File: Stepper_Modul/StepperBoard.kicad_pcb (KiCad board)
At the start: 2 copper layers, 55.1 x 100 mm, 67 parts, among them J101 Screw_Terminal_01x02, J102 Screw_Terminal_01x04, J103 Screw_Terminal_01x04, J104 Screw_Terminal_01x04, J105 Screw_Terminal_01x04, J106 Conn_02x20_Odd_Even, SW201 SW_DIP_x03, SW401 SW_DIP_x03, SW501 SW_DIP_x03, SW502 SW_DIP_x03, U201 TMC2226, U401 TMC2226, U501 TMC2226, U502 TMC2226

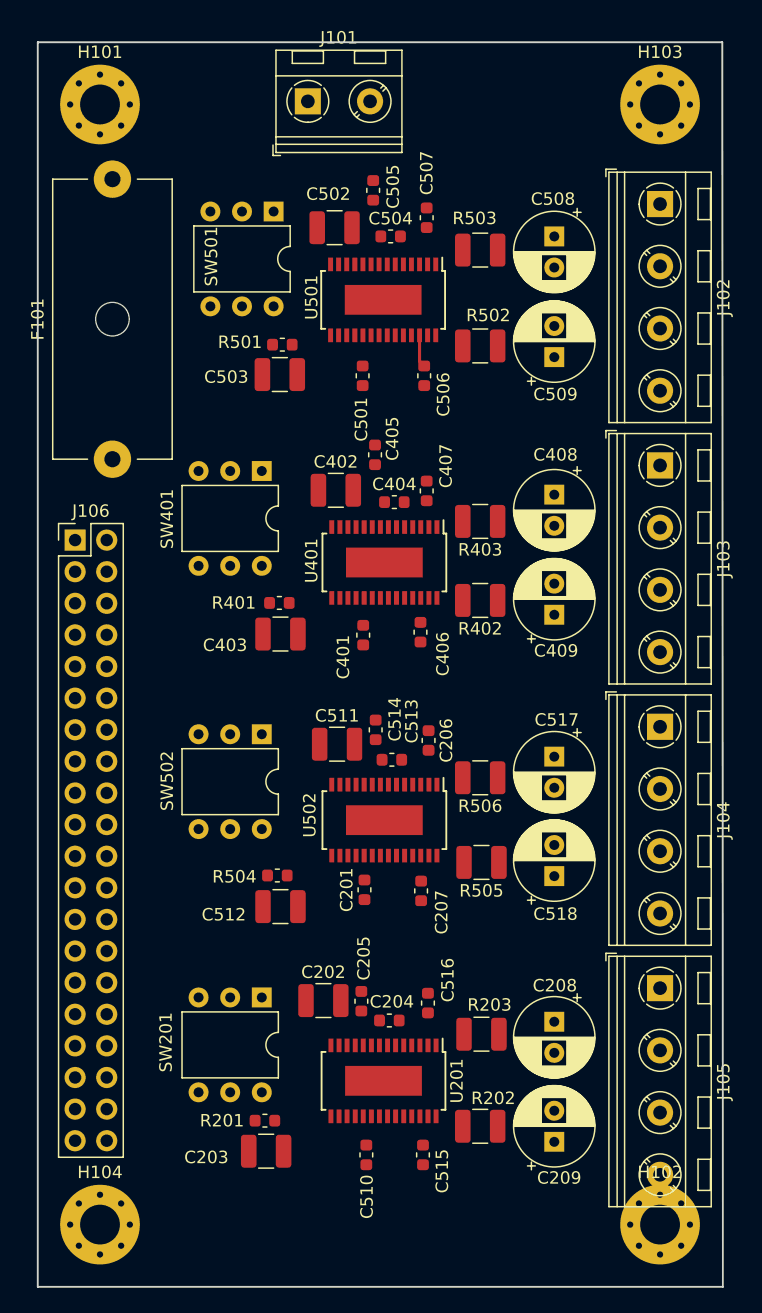
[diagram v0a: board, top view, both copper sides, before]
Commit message: stepper board fertig gestellt
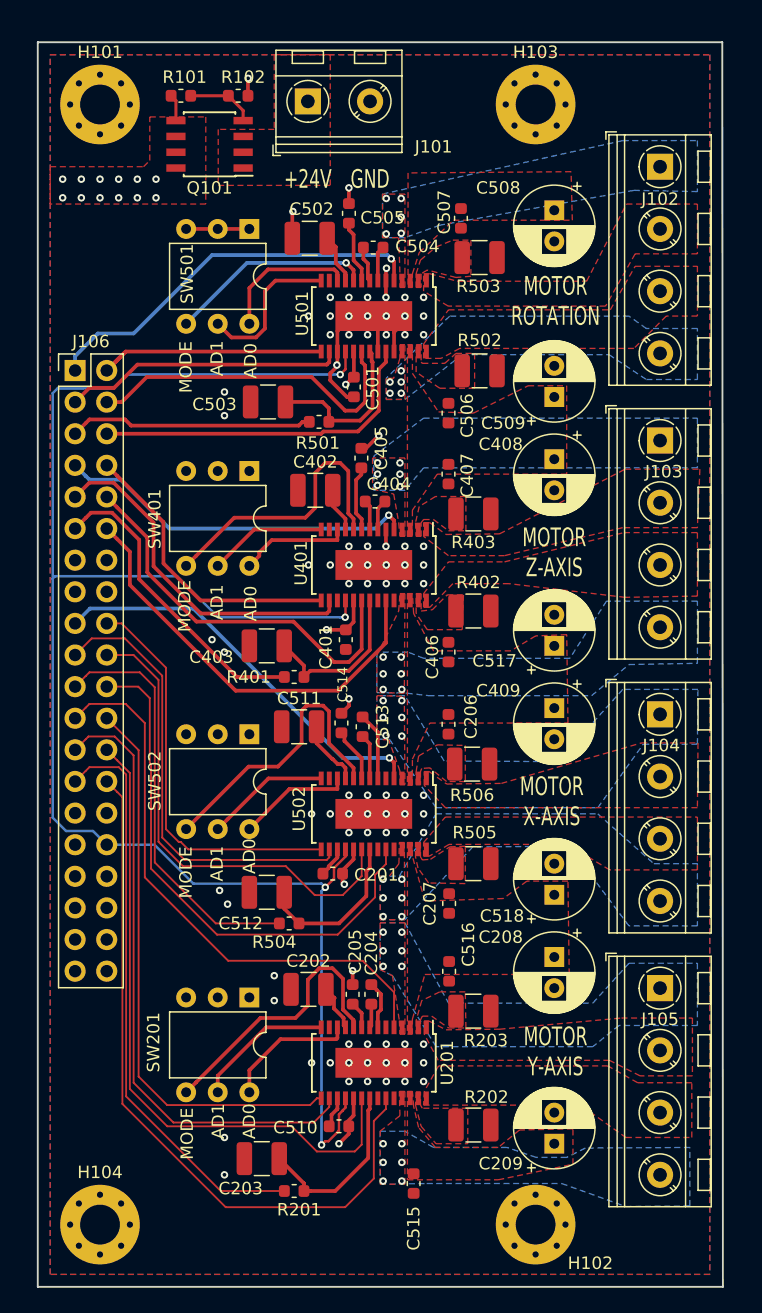
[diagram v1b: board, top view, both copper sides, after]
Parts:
- removed F101: Fuse, Fuse:Fuseholder_Cylinder-5x20mm_Schurter_0031_8201_Horizontal_Open
- added Q101: Si4431CDY, Package_SO:SOIC-8_3.9x4.9mm_P1.27mm, F.Cu at (93.8, 58.2)
- added R101: 22K1, Resistor_SMD:R_0603_1608Metric, F.Cu at (91.5, 54.3)
- added R102: 22K1, Resistor_SMD:R_0603_1608Metric, F.Cu at (96.1, 54.3)
- R201, R401, R501, R504: value 22k -> 22K1
- moved J106 13.6 mm to (83.0, 76.4)
- moved H102 10.0 mm to (120.0, 145.0)
- moved H103 10.0 mm to (120.0, 55.0)
- moved R501 6.87 mm to (102.6, 80.5)
- moved R201 6.12 mm to (100.6, 142.3)
- moved R401 6.07 mm to (100.6, 101.0)
- moved C208 5.20 mm to (121.5, 123.5)
- moved R504 3.97 mm to (100.2, 120.8)
- moved C517 3.90 mm to (121.5, 103.5)
- moved C506 3.58 mm to (113.0, 79.8), turned to 270 degrees
- moved C513 3.54 mm to (106.1, 105.0), turned to 90 degrees
- moved C511 3.36 mm to (101.0, 105.0)
- moved C509 3.20 mm to (121.5, 78.5)
- moved C510 3.18 mm to (104.2, 137.1), turned to 0 degrees
- moved C516 3.06 mm to (113.0, 124.7), turned to 90 degrees
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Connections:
- J101 pad 1: GND -> Net-(J101-Pad1)
- J101 pad 2: Net-(F101-Pad2) -> GND
- J106 pad 1: /CUR_ROT -> /EN_ROT
- J106 pad 10: /INDEX_Z -> /STEP_Z
- J106 pad 11: /EN_ROT -> /CUR_Z
- J106 pad 12: /EN_Z -> /DIR_Z
- J106 pad 17: /CUR_Y -> /EN_X
- J106 pad 18: /CUR_X -> /DIAG_X
- J106 pad 19: /STEP_Y -> /INDEX_X
- J106 pad 2: /CUR_Z -> /DIAG_ROT
- J106 pad 21: /DIR_Y -> /CUR_X
- J106 pad 23: /DIAG_Y -> /EN_Y
- J106 pad 24: /DIAG_X -> /DIAG_Y
- J106 pad 26: /INDEX_X -> /STEP_Y
- J106 pad 27: /EN_Y -> /CUR_Y
- J106 pad 28: /EN_X -> /DIR_Y
- J106 pad 3: /STEP_ROT -> /INDEX_ROT
- J106 pad 4: /STEP_Z -> /STEP_ROT
- J106 pad 5: /DIR_ROT -> /CUR_ROT
- J106 pad 6: /DIR_Z -> /DIR_ROT
- J106 pad 7: /DIAG_ROT -> /EN_Z
- J106 pad 9: /INDEX_ROT -> /INDEX_Z
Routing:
- net +3V3: track 0.00 -> 163.2 mm, vias 0 -> 4
- net /SINGLE_WIRE: track 0.00 -> 139.6 mm, vias 0 -> 4
- net /DIR_Y: track 0.00 -> 57.9 mm
- net /STEP_Y: track 0.00 -> 52.7 mm
- net /INDEX_Y: track 0.00 -> 50.3 mm
- net /CUR_Y: track 0.00 -> 46.5 mm
- net /EN_Y: track 0.00 -> 45.8 mm
- net /DIAG_Y: track 0.00 -> 45.7 mm
- net /DIR_X: track 0.00 -> 43.3 mm
- net /STEP_X: track 0.00 -> 38.9 mm
- net /INDEX_X: track 0.00 -> 36.7 mm
- net /DIR_Z: track 0.00 -> 34.4 mm
- net /CUR_X: track 0.00 -> 33.5 mm
- net /EN_X: track 0.00 -> 32.5 mm, vias 0 -> 1
- net /DIAG_X: track 0.00 -> 32.4 mm
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- added copper zone on F.Cu, net +24V
- added copper zone on In2.Cu, net +24V
- added copper zone on F.Cu, net /Stepper_rotation/OA1_ROT
- added copper zone on B.Cu, net /Stepper_rotation/OA2_ROT
- added copper zone on F.Cu, net /Stepper_rotation/OA2_ROT
- added copper zone on F.Cu, net /Stepper_rotation/OB1_ROT
- added copper zone on B.Cu, net /Stepper_rotation/OB2_ROT
- added copper zone on F.Cu, net /Stepper_rotation/OB2_ROT
- added copper zone on F.Cu, net /Stepper_x/OA1_X
- added copper zone on B.Cu, net /Stepper_x/OA2_X
- added copper zone on F.Cu, net /Stepper_x/OA2_X
- added copper zone on F.Cu, net /Stepper_x/OB1_X
- added copper zone on B.Cu, net /Stepper_x/OB2_X
- added copper zone on F.Cu, net /Stepper_x/OB2_X
- added copper zone on F.Cu, net /Stepper_y/OA1_Y
- added copper zone on B.Cu, net /Stepper_y/OA2_Y
- added copper zone on F.Cu, net /Stepper_y/OA2_Y
- added copper zone on F.Cu, net /Stepper_y/OB1_Y
- added copper zone on B.Cu, net /Stepper_y/OB2_Y
- added copper zone on F.Cu, net /Stepper_y/OB2_Y
- added copper zone on F.Cu, net /Stepper_z/OA1_Z
- added copper zone on B.Cu, net /Stepper_z/OA2_Z
- added copper zone on F.Cu, net /Stepper_z/OA2_Z
- added copper zone on F.Cu, net /Stepper_z/OB1_Z
- added copper zone on B.Cu, net /Stepper_z/OB2_Z
- added copper zone on F.Cu, net /Stepper_z/OB2_Z
- added copper zone on B.Cu, net GND
- added copper zone on F.Cu, net GND
- added copper zone on In1.Cu, net GND
- added copper zone on F.Cu, net Net-(J101-Pad1)
- added copper zone on F.Cu, net Net-(R202-Pad2)
- added copper zone on F.Cu, net Net-(R203-Pad2)
- added copper zone on F.Cu, net Net-(R402-Pad2)
- added copper zone on F.Cu, net Net-(R403-Pad2)
- added copper zone on F.Cu, net Net-(R502-Pad2)
- added copper zone on F.Cu, net Net-(R503-Pad2)
- added copper zone on F.Cu, net Net-(R505-Pad2)
- added copper zone on F.Cu, net Net-(R506-Pad2)
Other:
- copper layers 2 -> 4
- net class Default: clearance 0.2 -> 0.15; trace_width 0.25 -> 0.15; via_dia 0.8 -> 0.6; via_drill 0.4 -> 0.3
- rule trace_clearance: 0.2 -> 0.15
- rule trace_min: 0.2 -> 0.15
- rule via_min_size: 0.4 -> 0.3
- board text added: "+24V"
- board text added: "AD0"
- board text added: "AD1"
- board text added: "GND"
- board text added: "MODE"
- board text added: "MOTOR ROTATION"
- board text added: "MOTOR X-AXIS"
- board text added: "MOTOR Y-AXIS"
- board text added: "MOTOR Z-AXIS"
